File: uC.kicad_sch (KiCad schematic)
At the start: 16 parts, among them J3 Conn_01x04, J4 Conn_01x05, U3 STM32G431KBT6, U4 LSF0102DCUR, Y1 ECS-2520MV-xxx-xx

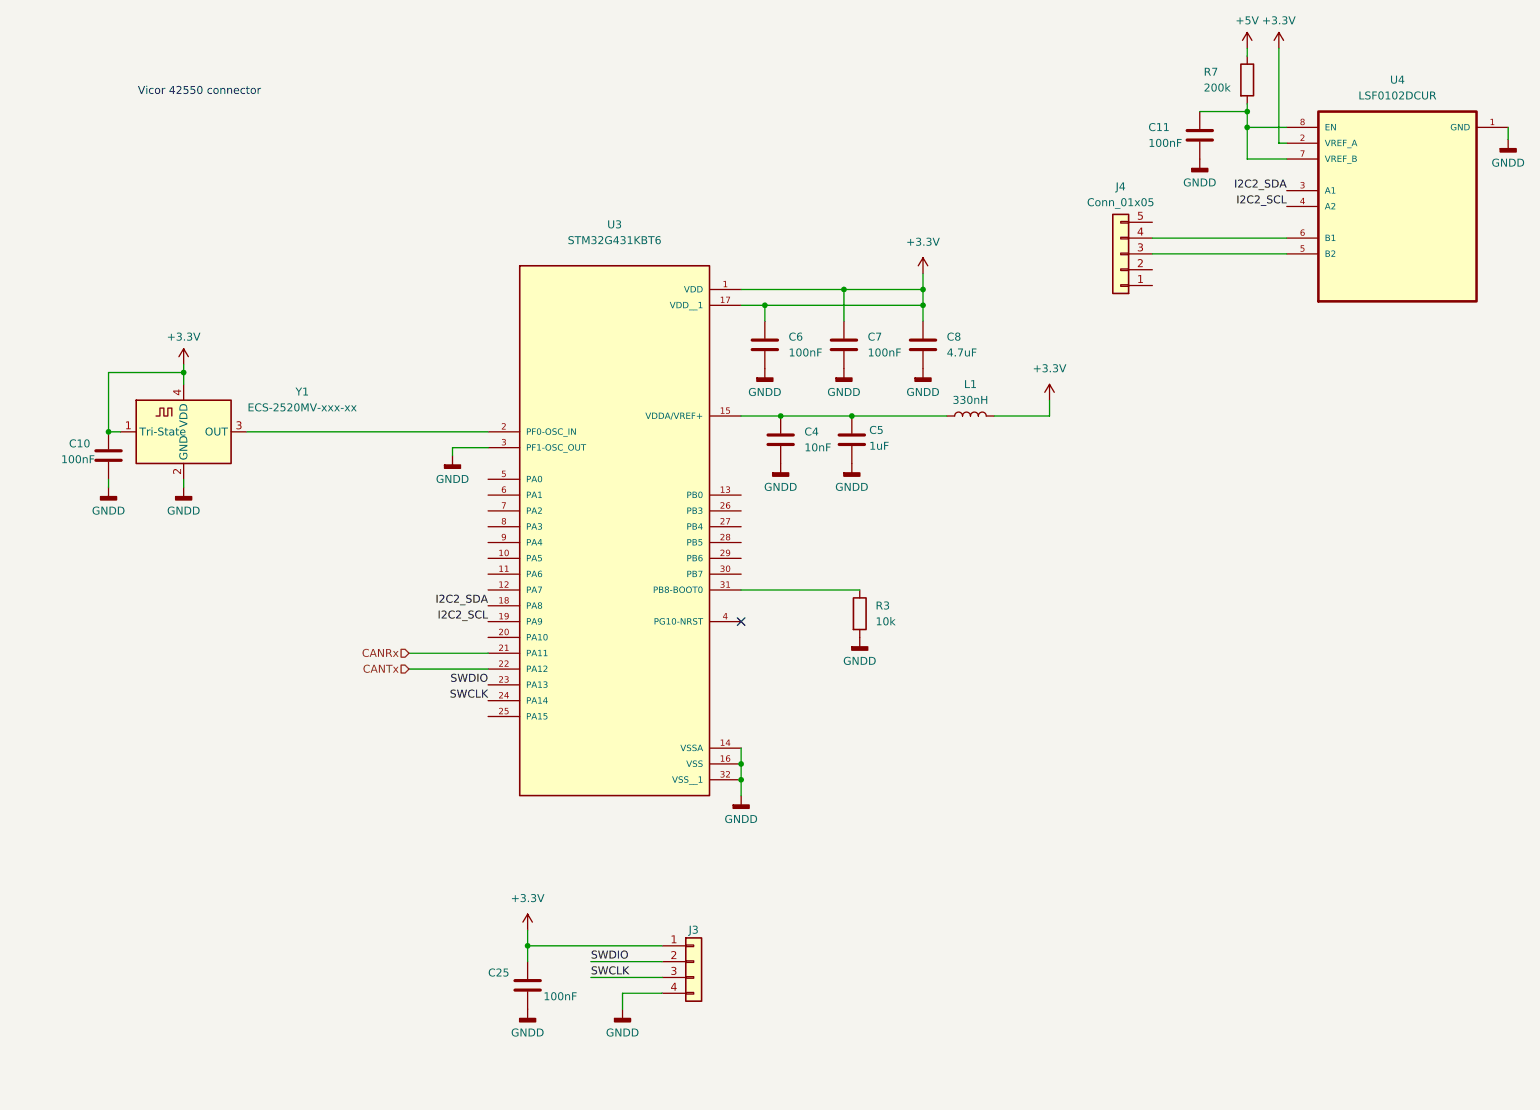
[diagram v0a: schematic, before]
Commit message: made todo, added power
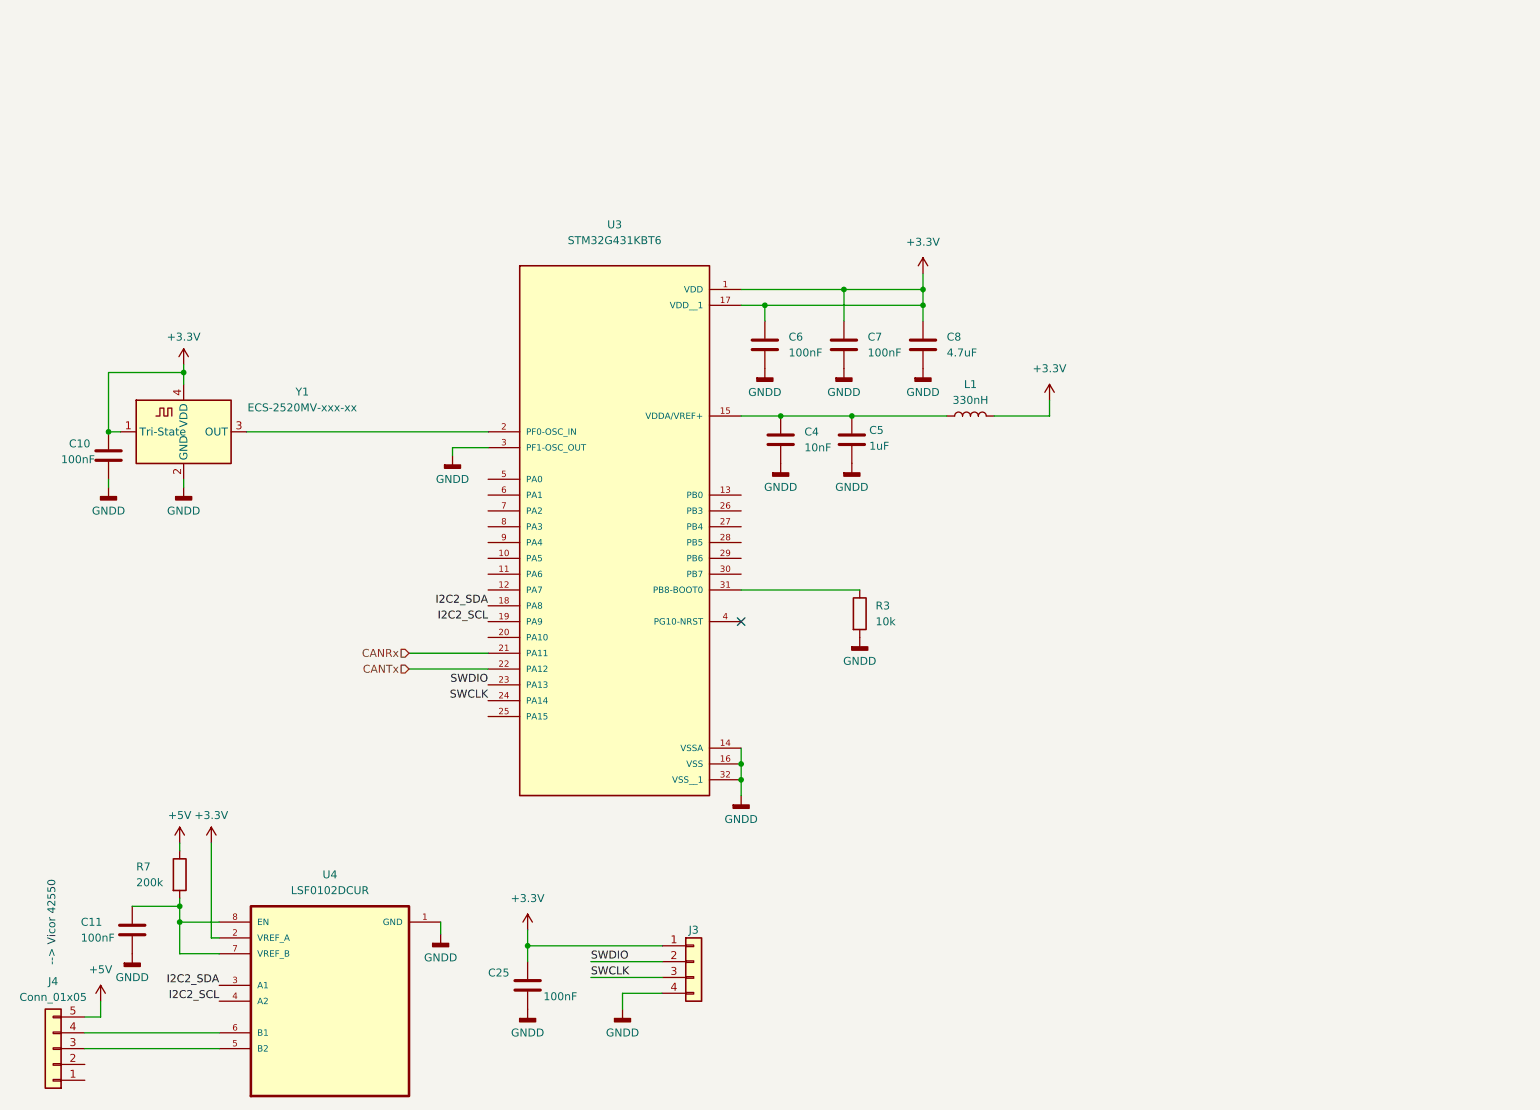
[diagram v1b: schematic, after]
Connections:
- net +5V: now also J4.5 (Pin_5)
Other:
- note added: "--> Vicor 42550"
- note removed: "Vicor 42550 connector"
- moved on the sheet: C11, J4, R7, U4
